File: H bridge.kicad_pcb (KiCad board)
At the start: 2 copper layers, 97 x 50 mm, 44 parts, among them J1 Fan, J2 5v Output, J3 Motor Terminal, J4 24v Power Input, J5 Control, Q1 IRLZ44N, Q2 IRLZ44N, Q3 IRLZ44N, Q4 IRLZ44N, SW1 SW_SPST, U1 IR2110, U2 IR2110, U3 LM7815_TO220, U4 LM7805_TO220

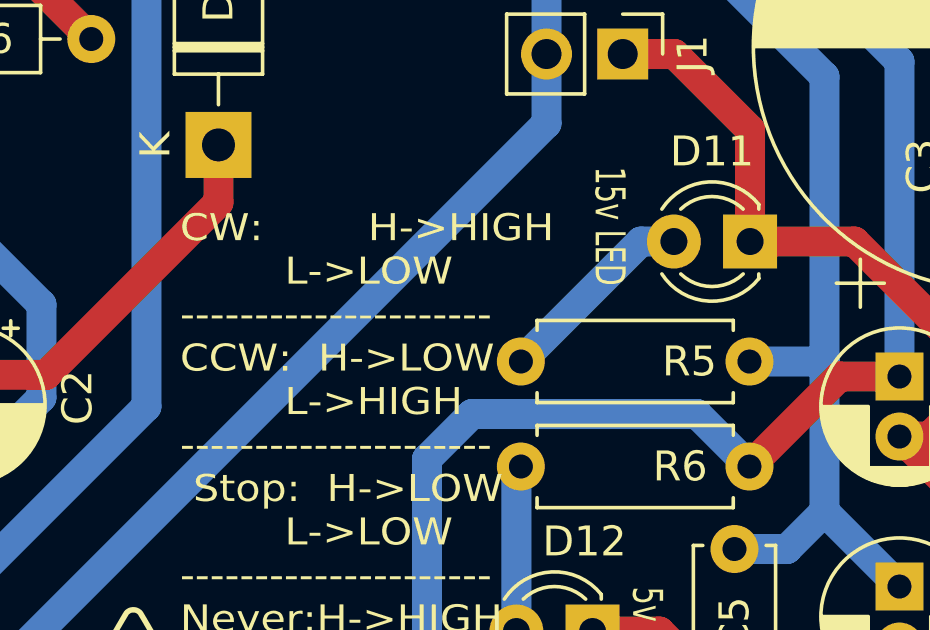
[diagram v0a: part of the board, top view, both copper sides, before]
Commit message: this is v2.0 it has the IC IR2110. (not tested yet).
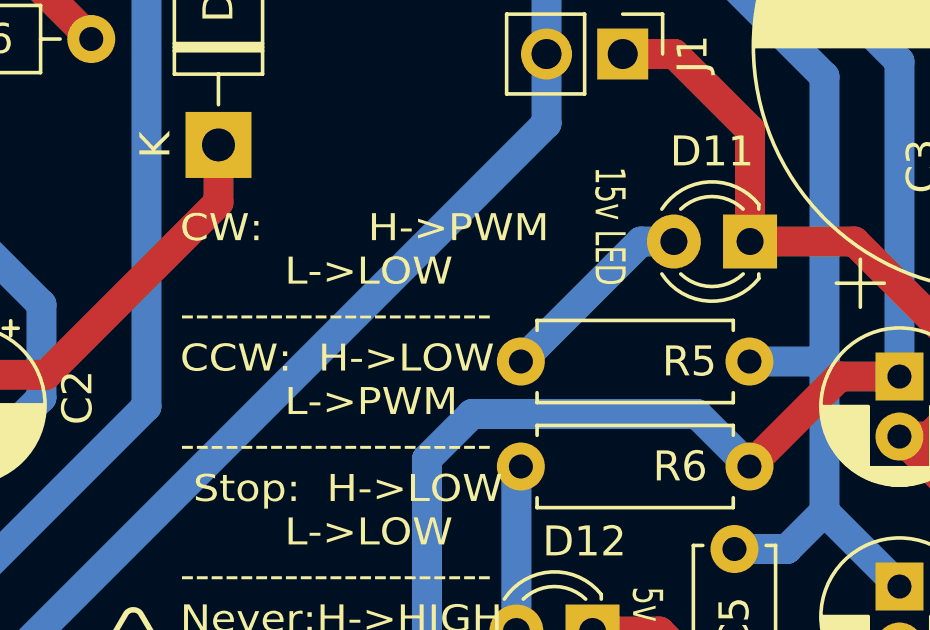
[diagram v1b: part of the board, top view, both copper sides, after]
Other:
- board text added: "CW: H->PWM L->LOW --------------------- CCW: H->LOW L->PWM --------------------- Stop: H->LOW L->LOW --------------------- Never:H->HIGH L->HIGH"
- board text removed: "CW: H->HIGH L->LOW --------------------- CCW: H->LOW L->HIGH --------------------- Stop: H->LOW L->LOW --------------------- Never:H->HIGH L->HIGH"
